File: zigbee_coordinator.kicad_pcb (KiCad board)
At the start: 2 copper layers, 33.5 x 33.5 mm, 51 parts, among them J1 USB_C_Receptacle_USB2.0, J10 CONN_POGO, J11 CONN_POGO, J12 SWD_HOLES, J13 UART_HOLES, J2 VCC_SEL, J3 SWD_PADS, J4 UART_PADS, J5 CONN_POGO, J6 CONN_POGO, J7 CONN_POGO, J8 CONN_POGO, J9 CONN_POGO, U1 93LCxxBxxOT, U2 MCP1603-OS, U3 FT232H, U4 74LVC126A, U5 74LVC126A, U6 TPS22917DBV, Y1 12MHz

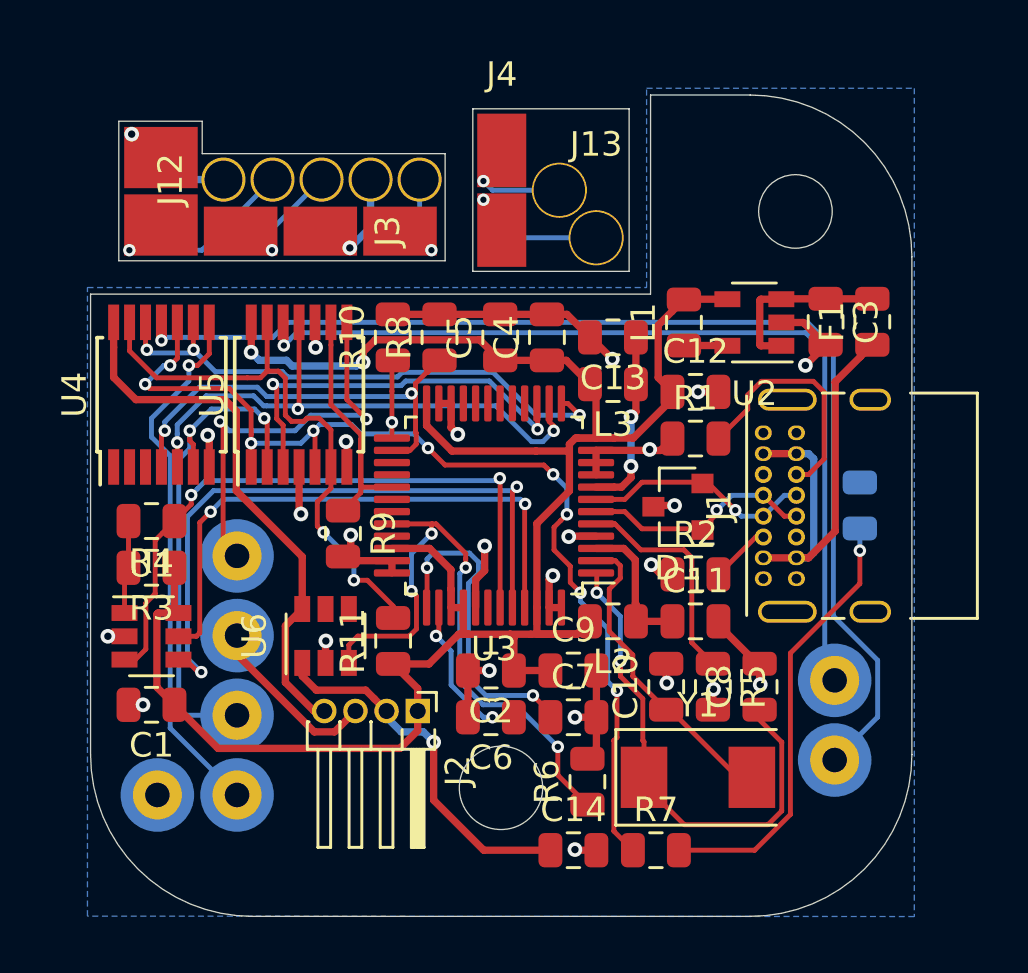
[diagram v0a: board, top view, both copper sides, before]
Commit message: Finalize
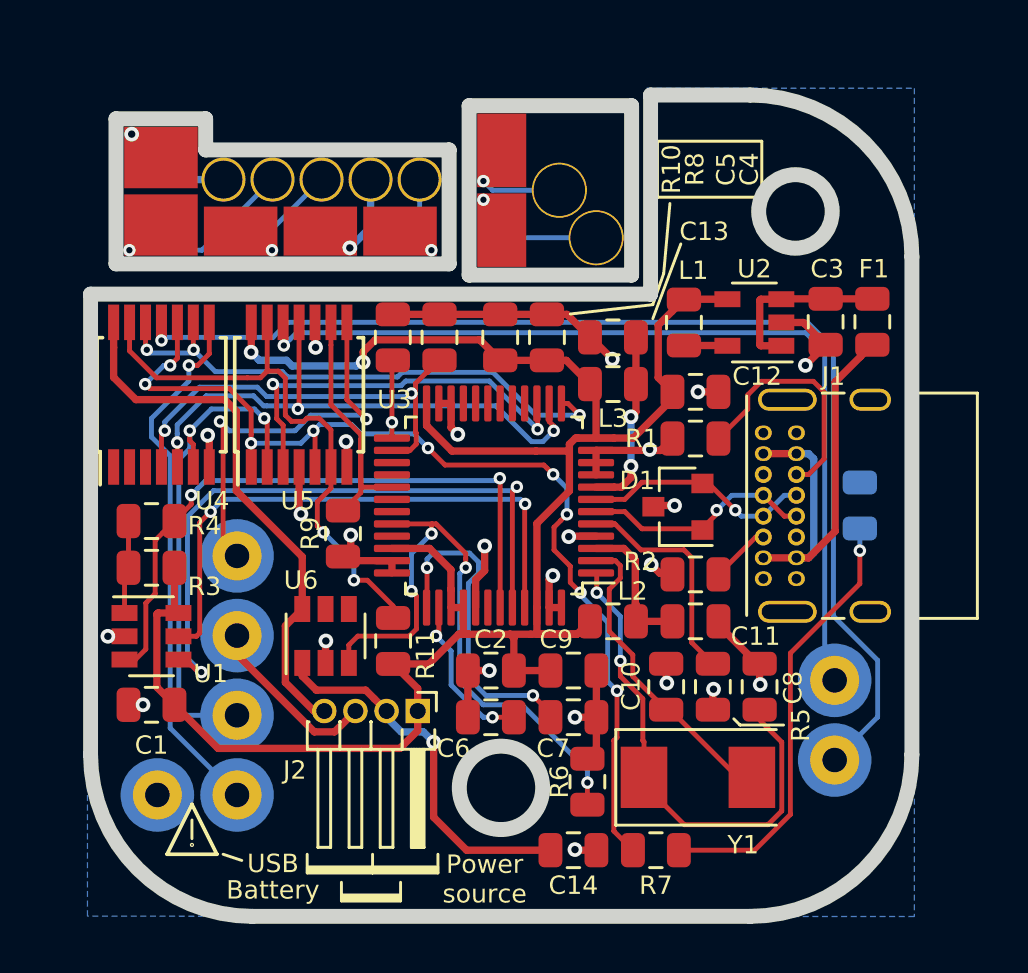
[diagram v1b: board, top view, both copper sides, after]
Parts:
- added G***: LOGO, tradfree_logo:tradfree_logo, B.Cu at (107.6, 114.0)
- added REF**: OSHW-Logo2_9.8x8mm_SilkScreen, Symbol:OSHW-Logo2_9.8x8mm_SilkScreen, B.Cu at (114.7, 125.3)
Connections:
- J1 pad A8: (no net) -> Net-(J1-PadA8)
- J1 pad B8: (no net) -> Net-(J1-PadB8)
- U3 pad 16: (no net) -> /~CTS~_TMS
- U3 pad 17: (no net) -> Net-(U3-Pad17)
- U3 pad 18: (no net) -> Net-(U3-Pad18)
- U3 pad 19: (no net) -> Net-(U3-Pad19)
- U3 pad 20: (no net) -> Net-(U3-Pad20)
- U3 pad 21: (no net) -> Net-(U3-Pad21)
- U3 pad 27: (no net) -> Net-(U3-Pad27)
- U3 pad 28: (no net) -> Net-(U3-Pad28)
- U3 pad 30: (no net) -> Net-(U3-Pad30)
- U3 pad 31: (no net) -> Net-(U3-Pad31)
- U3 pad 33: (no net) -> Net-(U3-Pad33)
- U3 pad 42: (no net) -> Net-(U3-Pad42)
- U4 pad 1: (no net) -> Net-(U4-Pad1)
- U4 pad 2: (no net) -> Net-(U4-Pad2)
- U4 pad 3: (no net) -> Net-(U4-Pad3)
- U6 pad 4: (no net) -> Net-(U6-Pad4)
- U6 pad 5: (no net) -> Net-(U6-Pad5)
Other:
- outline, holes or cut-outs redrawn
- board text added: "Battery"
- board text added: "Designed by corna & the TRÅDFREE team https://github.com/tradfree-mod"
- board text added: "Licensed under CERN-OHL-W v.2"
- board text added: "Power source"
- board text added: "TRÅDFREE"
- board text added: "USB"
